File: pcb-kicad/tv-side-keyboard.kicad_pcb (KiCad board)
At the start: 2 copper layers, 118 x 68 mm, 82 parts, among them J1 ESPProg-Port, J2 ESPProg-Port, J3 Keyboard USB, SW1 SW_Push, SW10 SW_Push, SW11 SW_Push, SW12 SW_Push, SW2 SW_Push, SW3 SW_Push, SW4 SW_Push, SW5 SW_Push, SW6 SW_Push, SW7 SW_Push, SW8 SW_Push, SW9 SW_Push, U1 joystick-b10k, U2 ESP32-C3-WROOM-02, U3 CH217K, U4 CH9329, U5 Regulator_AMS117-3.3, U6 CH32V003F4P6

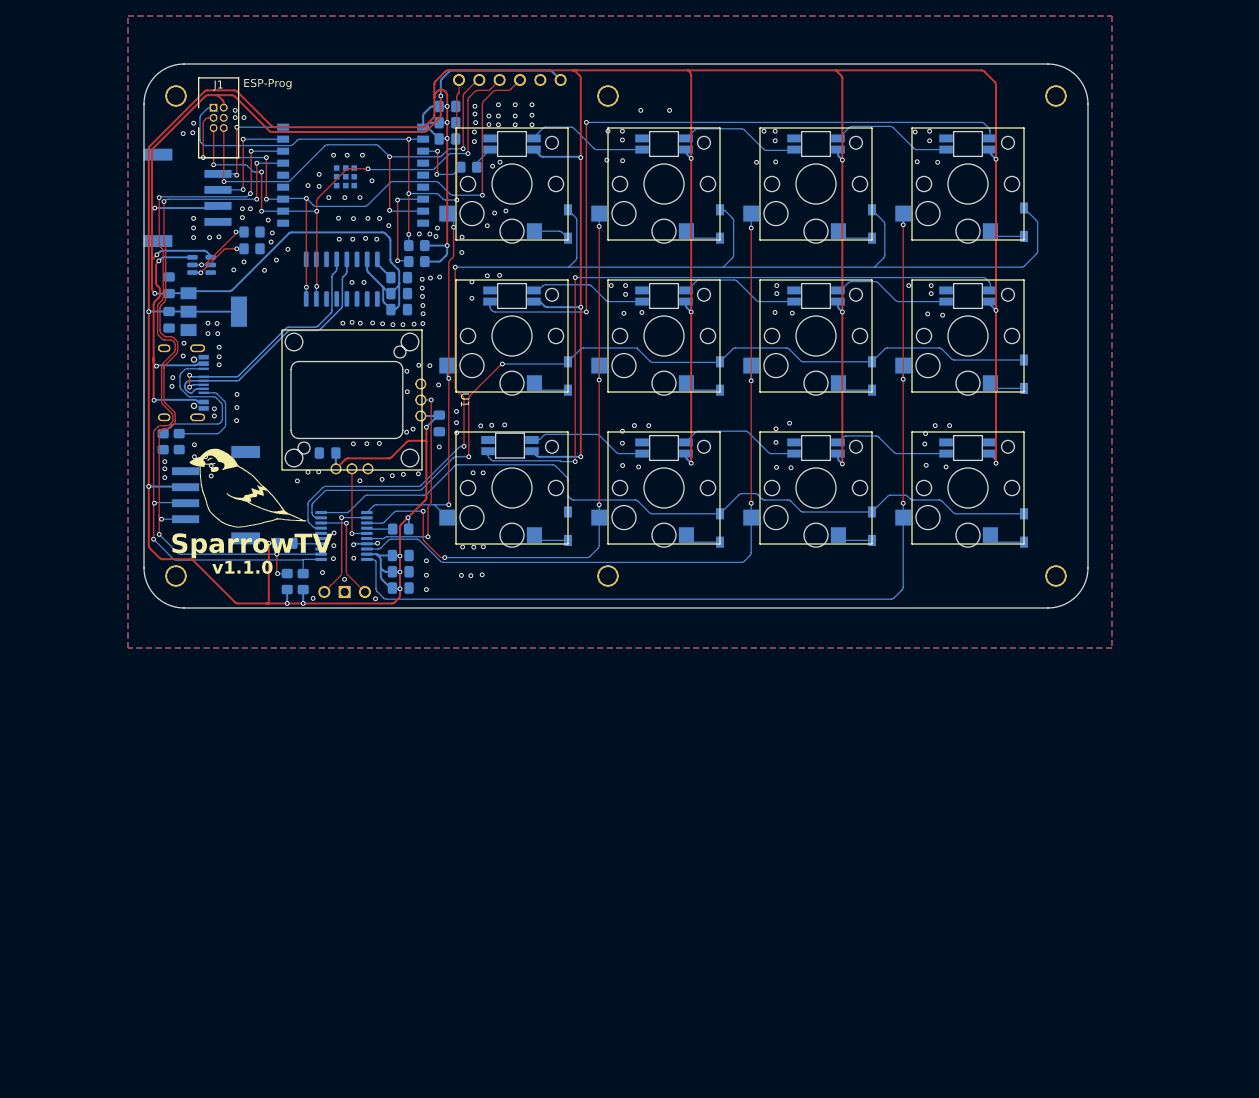
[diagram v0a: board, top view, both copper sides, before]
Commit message: wip
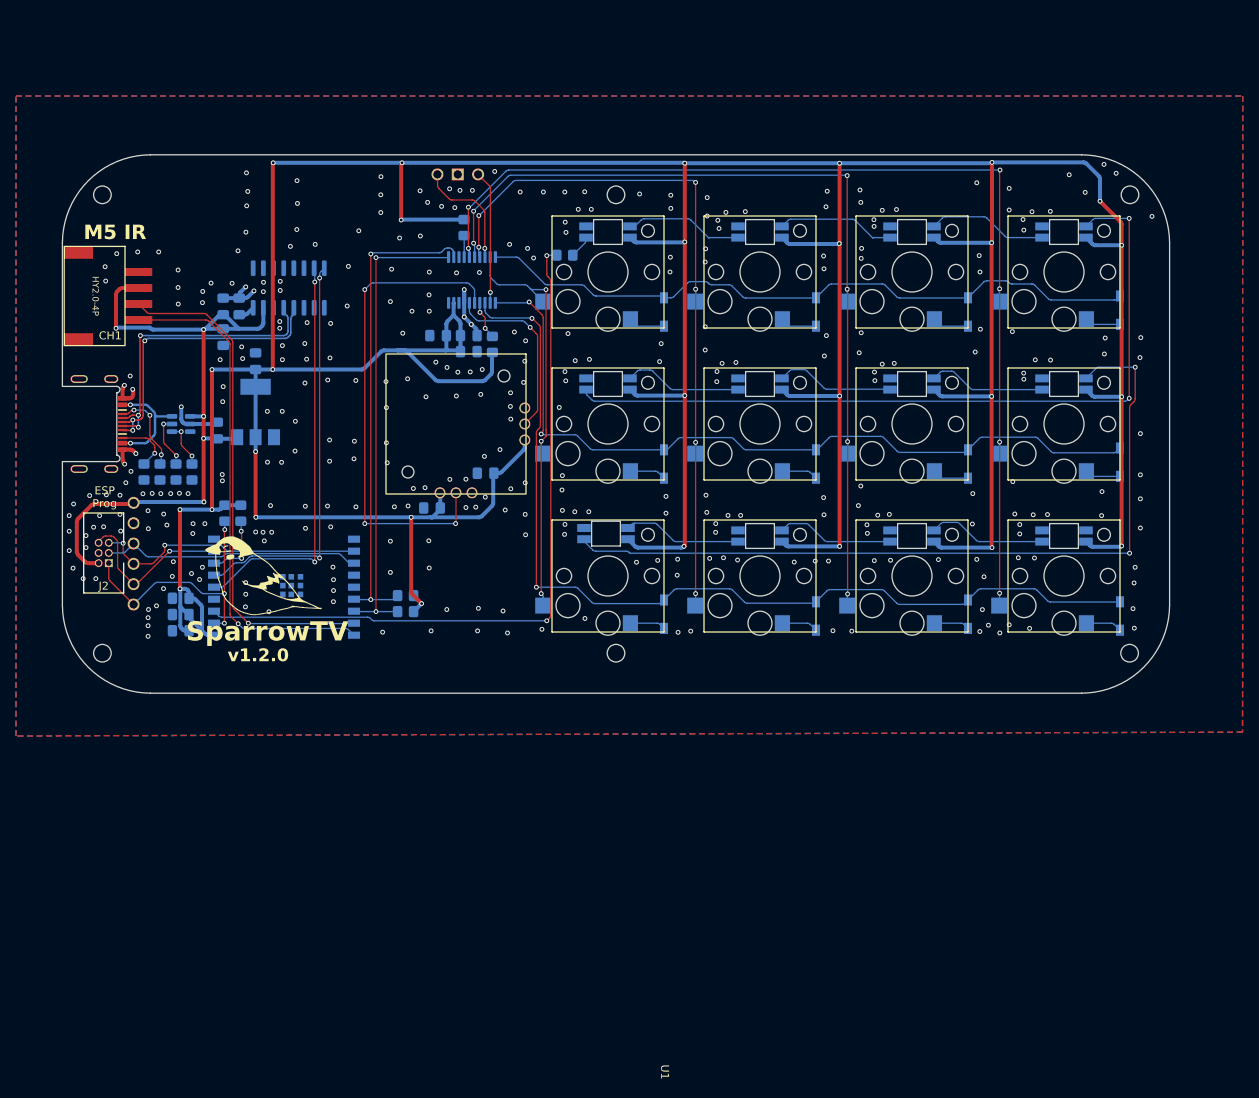
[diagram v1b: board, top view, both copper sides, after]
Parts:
- removed the CH2 at (58.2, 83.9)
- removed H1, H2, H3, H4, H5, H6: M2_v2, $sparrow62:M2_v2
- removed the REF** at (79.0, 72.0)
- added M2: M2-Hole, $74th:M2-Hole, F.Cu at (112.0, 46.4)
- added M2: M2-Hole, $74th:M2-Hole, F.Cu at (47.8, 103.7)
- added M2: M2-Hole, $74th:M2-Hole, F.Cu at (176.2, 46.4)
- added M2: M2-Hole, $74th:M2-Hole, F.Cu at (47.8, 46.4)
- added M3: M2-Hole, $74th:M2-Hole, F.Cu at (112.0, 103.7)
- added M4: M2-Hole, $74th:M2-Hole, F.Cu at (176.2, 103.7)
- added REF**: iphone-se-2_outline, $sparrow62:iphone-se-2_outline, F.Cu at (112.0, 75.0)
- added REF**: JLCJLCJLCJLC, $74th:JLCJLCJLCJLC, B.Cu at (166.8, 42.3)
- CH1: moved to F.Cu
- J1: renamed from J3; footprint $74th:USB-C-12-Pin-SMD -> $74th:USB-C-12-Pin-MidMount-ali-v5; moved to F.Cu
- moved J3 75.1 mm to (51.7, 84.9), turned to -90 degrees
- moved C13 73.5 mm to (57.6, 100.8), turned to 180 degrees
- moved C12 69.9 mm to (57.6, 98.8), turned to 180 degrees
- moved C11 66.4 mm to (57.6, 96.8), turned to 180 degrees
- moved J2 56.3 mm to (48.0, 91.1), turned to 180 degrees
- moved CH2 53.0 mm to (89.7, 43.8), turned to -90 degrees
- moved U6 52.4 mm to (70.5, 95.5), turned to 0 degrees
- moved R1 45.4 mm to (93.0, 50.5), turned to -90 degrees
- moved G*** 41.2 mm to (95.9, 99.3)
- moved R9 41.2 mm to (63.1, 86.2), turned to -90 degrees
- moved R8 38.4 mm to (65.1, 86.2), turned to -90 degrees
- moved U2 35.8 mm to (94.0, 57.0), turned to 90 degrees
- moved R5 31.5 mm to (57.0, 81.0), turned to -90 degrees
- moved C6 30.8 mm to (93.6, 66.0)
- moved C4 29.9 mm to (89.8, 64.0), turned to 180 degrees
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- renumbered C4 to C1, C3 to C11, C2 to C12, C1 to C13, C7 to C2, C11 to C3, C12 to C4, C6 to C5, C13 to C6, C8 to C7, C5 to C8, CH3 to CH2, J1 to J2, J2 to J3, R9 to R1, R11 to R10, R10 to R11, R1 to R2, R8 to R3, R2 to R5, R5 to R8, R3 to R9, U6 to U2, U4 to U3, U5 to U4, U3 to U5, U2 to U6
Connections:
- J2 pad 3: /CH9329_RXD -> /ESP32C3_TXD
- J2 pad 5: /CH9329_TXD -> /ESP32C3_RXD
- J3 pad 3: /CH9329_RXD -> /ESP32C3_TXD
- J3 pad 4: /CH9329_TXD -> /ESP32C3_RXD
- U2 pad 1: /COL1 -> /ROW2
- U2 pad 10: /COL4 -> unconnected-(U6-PC0-Pad10)
- U2 pad 15: unconnected-(U6-PC5/SPI_SCK-Pad15) -> /COL4
- U2 pad 16: unconnected-(U6-PC6/SPI_MOSI-Pad16) -> /COL3
- U2 pad 17: /ROW1 -> /COL2
- U2 pad 19: /ROW2 -> /COL1
- U2 pad 20: /ROW3 -> /ROW1
- U2 pad 3: /COL2 -> /ROW3
- U2 pad 8: /COL3 -> unconnected-(U6-PD0-Pad8)
- U6 pad 11: /CH9329_TXD -> /ESP32C3_RXD
- U6 pad 12: /CH9329_RXD -> /ESP32C3_TXD
- U6 pad 5: unconnected-(U2-GPIO6-Pad5) -> /CH9329_TXD
- U6 pad 6: unconnected-(U2-GPIO7-Pad6) -> /CH9329_RXD
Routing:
- net /LED: track 8.10 -> 89.3 mm
- net /ROW1: track 154.2 -> 84.6 mm, vias 2 -> 0
- net +5V: track 151.3 -> 85.4 mm, vias 4 -> 5
- net +3.3V: track 551.1 -> 608.3 mm, vias 26 -> 28
- net /YOUT: track 9.97 -> 60.5 mm, vias 1 -> 3
- net /IR_IN: track 14.2 -> 63.1 mm, vias 2 -> 1
- net /IR_OUT: track 14.5 -> 62.3 mm, vias 2 -> 1
- net /ESP32C3_BOOT: track 59.7 -> 20.4 mm, vias 4 -> 1
- net /SDA: track 95.9 -> 58.7 mm, vias 5 -> 2
- net /ESP32C3_RST: track 68.9 -> 33.5 mm, vias 4 -> 3
- net /ESP32C3_RXD: track 0.00 -> 34.1 mm, vias 0 -> 2
- net /SCL: track 93.5 -> 59.6 mm, vias 7 -> 2
- net /ESP32C3_TXD: track 0.00 -> 31.8 mm
- net /CH9329_RXD: track 78.2 -> 50.6 mm, vias 6 -> 2
- net GND: track 3.08 -> 27.3 mm, vias 208 -> 352
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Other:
- board size 118 x 68 mm -> 138.4 x 67.3 mm
- board text added: "ESP Prog"
- board text added: "TXD"
- board text added: "v1.2.0"
- board text removed: "DTX"
- board text removed: "ESP-Prog"
- board text removed: "JoyPoint"
- board text removed: "v1.1.0"

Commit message: iphone se 2 sized
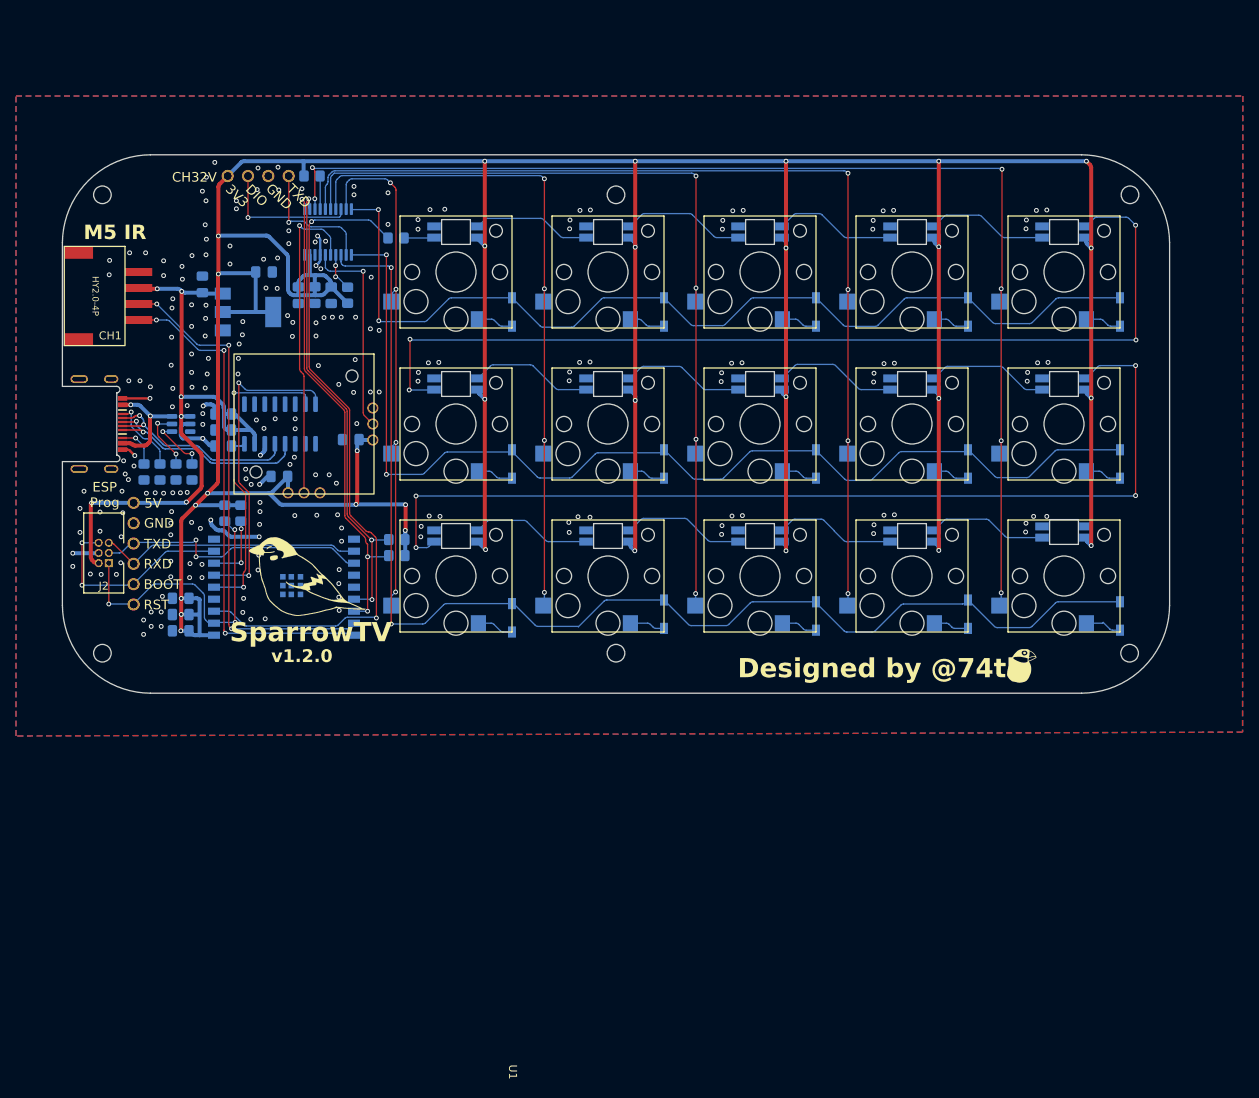
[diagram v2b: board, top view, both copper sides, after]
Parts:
- added D1: 1N4148W, $sparrow62:D3_SMD_v2, F.Cu at (99.0, 61.0)
- added D15: 1N4148W, $sparrow62:D3_SMD_v2, F.Cu at (99.0, 99.2)
- added D20: SK6812MINI, $74th:YS-SK6812MINI-E-BACK-RIGHT, B.Cu at (92.0, 51.0)
- added D25: SK6812MINI, $74th:YS-SK6812MINI-E-BACK-RIGHT, B.Cu at (92.0, 70.0)
- added D30: SK6812MINI, $74th:YS-SK6812MINI-E-BACK-RIGHT, B.Cu at (92.0, 89.0)
- added D6: 1N4148W, $sparrow62:D3_SMD_v2, F.Cu at (99.0, 80.0)
- added MISC-ICON: LOGO, 74th:Logo_74th_5mm, F.Cu at (162.6, 105.5)
- added SW1: SW_Push, $sparrow62:Choc_1Side_1.0u, F.Cu at (92.0, 56.0)
- added SW11: SW_Push, $sparrow62:Choc_1Side_1.0u, F.Cu at (92.0, 94.0)
- added SW6: SW_Push, $sparrow62:Choc_1Side_1.0u, F.Cu at (92.0, 75.0)
- CH2: footprint $74th:CH32V003-DebugPort -> 74th:PinOut_4Pin
- moved G*** 60.9 mm to (52.1, 57.0)
- moved CH2 26.2 mm to (63.5, 44.0), turned to 0 degrees
- moved C10 25.8 mm to (69.9, 81.5)
- moved R2 21.2 mm to (84.5, 51.8)
- moved R1 20.1 mm to (74.0, 44.0), turned to 0 degrees
- moved C4 19.9 mm to (74.3, 58.9), turned to -90 degrees
- moved R3 19.1 mm to (78.5, 58.9)
- moved U1 19.0 mm to (73.0, 75.0)
- moved U2 19.0 mm to (76.0, 51.0)
- moved C3 18.6 mm to (76.4, 58.9), turned to -90 degrees
- moved C2 18.4 mm to (60.3, 57.5)
- moved C5 18.2 mm to (72.3, 58.9), turned to -90 degrees
- moved C9 17.6 mm to (62.9, 77.8), turned to 180 degrees
- moved U4 17.0 mm to (70.0, 75.0)
- moved C7 15.5 mm to (62.9, 75.8), turned to 180 degrees
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- renumbered C7 to C1, C9 to C10, C8 to C2, C6 to C3, C3 to C4, C4 to C5, C5 to C6, C2 to C7, C10 to C8, C1 to C9, D5 to D10, D9 to D11, D10 to D12, D11 to D13, D12 to D14, D13 to D16, D14 to D17, D15 to D18, D16 to D19, D17 to D21, D18 to D22, D19 to D23, D20 to D24, D22 to D26, D23 to D27, D24 to D28, D21 to D29, D1 to D5, D6 to D7, D7 to D8, D8 to D9, M2 to M1, M2 to M3, M2 to M4, M3 to M5, M4 to M6, SW8 to SW10, SW9 to SW12, SW10 to SW13, SW11 to SW14, SW12 to SW15, SW1 to SW2, SW2 to SW3, SW3 to SW4, SW4 to SW5, SW5 to SW7, SW6 to SW8, SW7 to SW9, U4 to U3, U3 to U4
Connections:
- CH2 pad 1: /CH32V003_SWDIO -> +3.3V
- CH2 pad 2: GND -> /CH32V003_SWDIO
- CH2 pad 3: /CH32V003_TXD -> GND
- D16 pad 2: Net-(D13-DOUT) -> Net-(D16-DOUT)
- D19 pad 4: Net-(D16-DIN) (its old number) -> Net-(D19-DIN)
- D21 pad 2: Net-(D17-DOUT) -> Net-(D21-DOUT)
- D24 pad 4: Net-(D13-DOUT) -> Net-(D24-DIN)
- D29 pad 4: Net-(D17-DOUT) -> Net-(D29-DIN)
- R2 pad 1: Net-(D16-DIN) (its old number) -> Net-(D20-DIN)
- SW10 pad 1: /COL4 -> /COL5
- SW12 pad 1: /COL1 -> /COL2
- SW13 pad 1: /COL2 -> /COL3
- SW14 pad 1: /COL3 -> /COL4
- SW15 pad 1: /COL4 -> /COL5
- SW2 pad 1: /COL1 -> /COL2
- SW3 pad 1: /COL2 -> /COL3
- SW4 pad 1: /COL3 -> /COL4
- SW5 pad 1: /COL4 -> /COL5
- SW7 pad 1: /COL1 -> /COL2
- SW8 pad 1: /COL2 -> /COL3
- SW9 pad 1: /COL3 -> /COL4
- U2 pad 13: unconnected-(U6-PC3-Pad13) -> /COL5
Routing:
- net /COL5: track 0.00 -> 148.6 mm, vias 0 -> 6
- net Net-(D21-DOUT): track 0.00 -> 122.0 mm, vias 0 -> 4
- net Net-(D16-DOUT): track 0.00 -> 121.6 mm, vias 0 -> 4
- net Net-(D17-DOUT): track 99.1 -> 0.00 mm, vias 2 -> 0
- net Net-(D13-DOUT): track 97.2 -> 0.00 mm, vias 2 -> 0
- net +3.3V: track 608.3 -> 549.9 mm, vias 28 -> 31
- net /ROW1: track 84.6 -> 122.4 mm, vias 0 -> 2
- net /ROW2: track 98.1 -> 134.9 mm
- net /ROW3: track 119.2 -> 154.7 mm
- net /YOUT: track 60.5 -> 40.2 mm, vias 3 -> 1
- net Net-(D24-DIN): track 0.00 -> 15.4 mm
- net Net-(D29-DIN): track 0.00 -> 15.0 mm
- net Net-(D19-DIN): track 0.00 -> 14.8 mm
- net /CH9329_TXD: track 50.8 -> 38.8 mm
- net /COL1: track 53.5 -> 65.1 mm, vias 3 -> 4
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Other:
- board text added: "3V3"
- board text added: "DIO"
- board text added: "Designed by @74th"
